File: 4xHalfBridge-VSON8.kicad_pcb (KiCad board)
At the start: 2 copper layers, 90 x 36 mm, 98 parts, among them U1 VSON8_Nexfet, U10 24LC01, U2 VSON8_Nexfet, U3 VSON8_Nexfet, U4 VSON8_Nexfet, U5 VSON8_Nexfet, U6 VSON8_Nexfet, U7 VSON8_Nexfet, U8 VSON8_Nexfet, U9 PowerStage_L

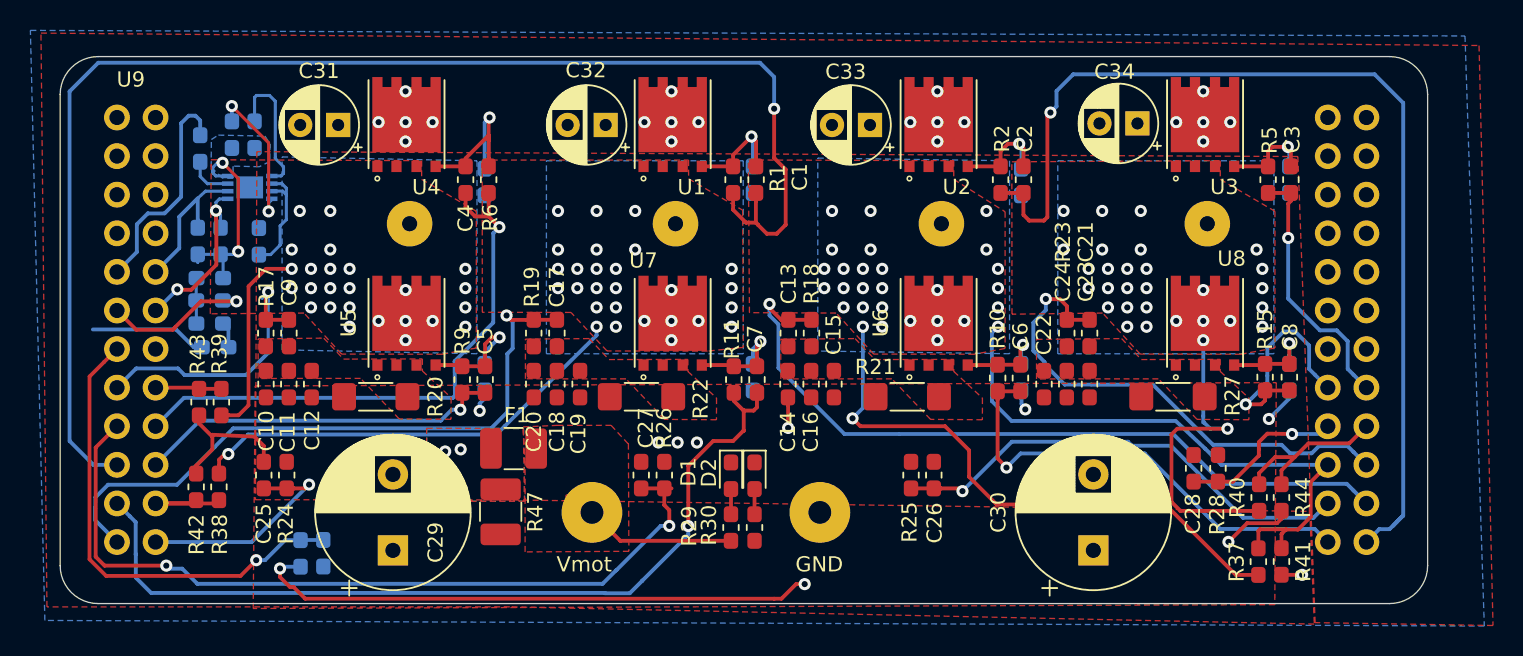
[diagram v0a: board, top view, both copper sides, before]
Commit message: add files
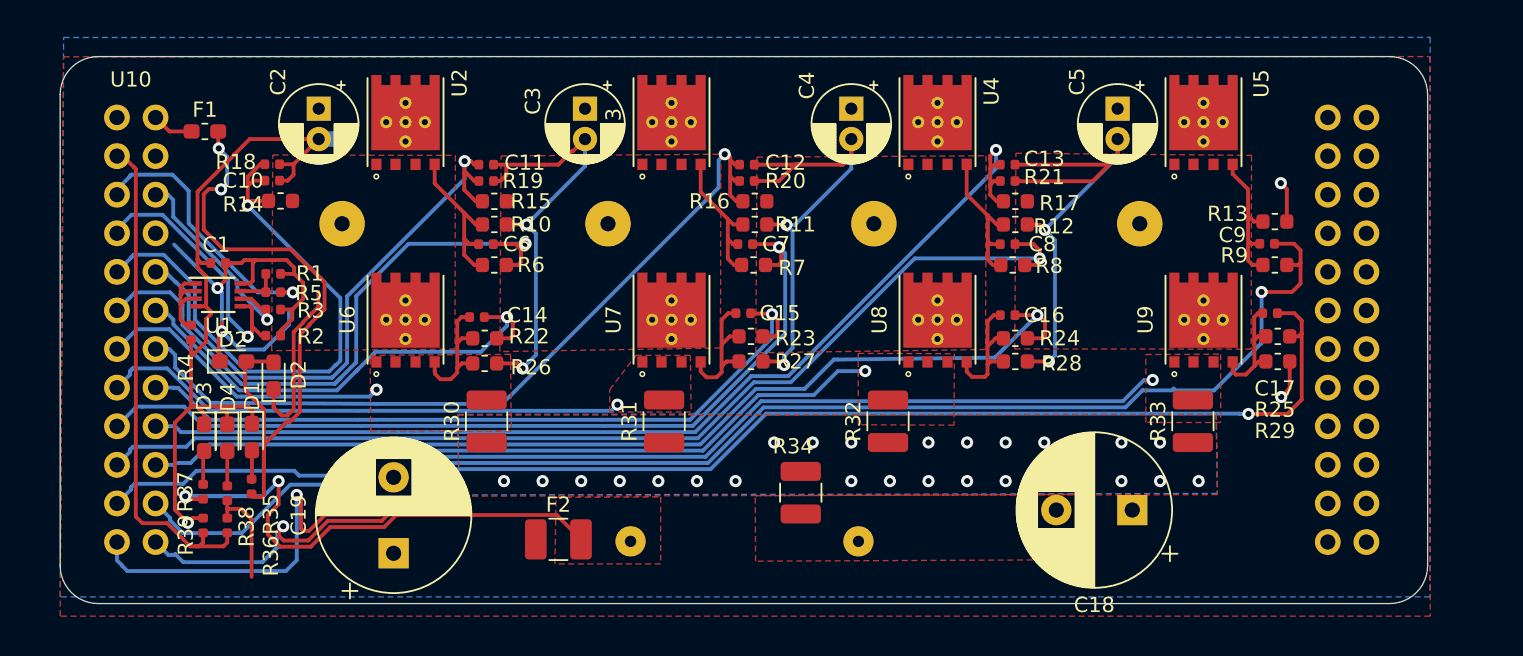
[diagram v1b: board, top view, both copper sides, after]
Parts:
- removed C20, C21, C22, C23, C24, C25, C26, C27, C28: C, Capacitor_SMD:C_0603_1608Metric_Pad1.05x0.95mm_HandSolder
- removed C29, C30: CP, Capacitor_THT:CP_Radial_D10.0mm_P5.00mm
- removed C31, C32, C33, C34: CP, Capacitor_THT:CP_Radial_D5.0mm_P2.50mm
- removed C35: X7R, 47-nF, Capacitor_SMD:C_0603_1608Metric_Pad1.05x0.95mm_HandSolder
- removed the D2 at (45.7, 27.6)
- removed R40, R41, R42, R43, R44, R45, R46: R, Resistor_SMD:R_0603_1608Metric_Pad1.05x0.95mm_HandSolder
- removed R47: R, Resistor_SMD:R_1210_3225Metric_Pad1.42x2.65mm_HandSolder
- removed the U10 at (12.5, 8.61)
- added D2: D_Schottky, Diode_SMD:D_0603_1608Metric_Pad1.05x0.95mm_HandSolder, F.Cu at (14.0, 21.0)
- added D2: D_Schottky, Diode_SMD:D_0603_1608Metric_Pad1.05x0.95mm_HandSolder, F.Cu at (11.4, 20.1)
- added U9: VSON8_Nexfet, Custom_Mosfet:MOSFET_CSD19531Q5A, F.Cu at (75.2, 17.3)
- C1, C10, C11, C12, C13, C14, C15, C16, C17, C6, C7, C8, C9: footprint Capacitor_SMD:C_0603_1608Metric_Pad1.05x0.95mm_HandSolder -> Capacitor_SMD:C_0402_1005Metric
- C18, C19: value C -> CP; footprint Capacitor_SMD:C_0603_1608Metric_Pad1.05x0.95mm_HandSolder -> Capacitor_THT:CP_Radial_D10.0mm_P5.00mm
- C2, C3, C4, C5: footprint Capacitor_SMD:C_0603_1608Metric_Pad1.05x0.95mm_HandSolder -> Capacitor_THT:CP_Radial_D5.0mm_P2.00mm
- D3: moved to F.Cu
- D4: value D_Schottky -> LED; footprint Diode_SMD:D_0603_1608Metric_Pad1.05x0.95mm_HandSolder -> LED_SMD:LED_0603_1608Metric_Pad1.05x0.95mm_HandSolder; moved to F.Cu
- F1: footprint Fuse:Fuse_1210_3225Metric_Pad1.42x2.65mm_HandSolder -> Fuse:Fuse_0603_1608Metric_Pad1.05x0.95mm_HandSolder
- F2: footprint Fuse:Fuse_0603_1608Metric_Pad1.05x0.95mm_HandSolder -> Fuse:Fuse_1210_3225Metric_Pad1.42x2.65mm_HandSolder; moved to F.Cu
- R1, R18, R19, R2, R37, R38, R39, R5: value R -> R_Small; footprint Resistor_SMD:R_0603_1608Metric_Pad1.05x0.95mm_HandSolder -> Resistor_SMD:R_0402_1005Metric
- R10, R11, R15, R17, R23, R24, R25, R26, R28, R29, R6, R9: value R -> R_Small; footprint Resistor_SMD:R_0603_1608Metric_Pad1.05x0.95mm_HandSolder -> Resistor_SMD:R_0603_1608Metric
- R12, R13, R14, R16, R7, R8: value R -> R_Small; footprint Resistor_SMD:R_0603_1608Metric_Pad1.05x0.95mm_HandSolder -> Resistor_SMD:R_0603_1608Metric; moved to F.Cu
- R20, R21: value R -> R_Small; footprint Resistor_SMD:R_1806_4516Metric_Pad1.57x1.80mm_HandSolder -> Resistor_SMD:R_0402_1005Metric
- R22, R27: value R -> R_Small; footprint Resistor_SMD:R_1806_4516Metric_Pad1.57x1.80mm_HandSolder -> Resistor_SMD:R_0603_1608Metric
- R3, R35, R36, R4: value R -> R_Small; footprint Resistor_SMD:R_0603_1608Metric_Pad1.05x0.95mm_HandSolder -> Resistor_SMD:R_0402_1005Metric; moved to F.Cu
- R30: value R -> R_Small; footprint Resistor_SMD:R_0603_1608Metric_Pad1.05x0.95mm_HandSolder -> Resistor_SMD:R_1210_3225Metric
- R31, R32, R33, R34: value R -> R_Small; footprint Resistor_SMD:R_0603_1608Metric_Pad1.05x0.95mm_HandSolder -> Resistor_SMD:R_1210_3225Metric; moved to F.Cu
- U1: value VSON8_Nexfet -> 24LC01; footprint Custom_Mosfet:MOSFET_CSD19531Q5A -> Package_DFN_QFN:DFN-8-1EP_3x2mm_P0.5mm_EP1.75x1.45mm
- moved R37 69.6 mm to (9.41, 28.6)
- moved R5 65.9 mm to (14.0, 15.5), turned to 180 degrees
- moved R33 65.1 mm to (74.5, 24.0)
- moved C9 64.7 mm to (79.4, 12.3), turned to 180 degrees
- moved R4 55.5 mm to (8.61, 18.2)
- moved U5 54.1 mm to (75.2, 4.32)
- moved R9 54.0 mm to (79.9, 13.7), turned to 180 degrees
- moved R15 52.0 mm to (28.6, 9.53), turned to 180 degrees
- moved R17 50.1 mm to (62.9, 9.53), turned to 0 degrees
- moved R2 49.0 mm to (14.0, 18.4), turned to 180 degrees
- moved R24 48.8 mm to (62.9, 18.5), turned to 0 degrees
- moved C17 47.0 mm to (79.6, 16.9), turned to 180 degrees
- moved C3 46.7 mm to (34.5, 3.43)
- moved C2 46.6 mm to (17.0, 3.43)
- moved R32 45.8 mm to (54.5, 24.0)
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- renumbered U9 to U10
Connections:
- C1 pad 1: Net-(C1-Pad1) -> /CarrierBoard/5V
- C1 pad 2: /BHG -> GND
- C10 pad 2: Net-(C10-Pad2) -> /4xHalfBridge/VSENA
- C11 pad 2: Net-(C10-Pad2) -> /4xHalfBridge/VSENB
- C12 pad 2: Net-(C10-Pad2) -> /4xHalfBridge/VSENC
- C13 pad 1: Net-(C13-Pad1) -> GND
- C13 pad 2: /CISENP -> /4xHalfBridge/VSEND
- C14 pad 1: GND -> /4xHalfBridge/ALG
- C14 pad 2: Net-(C13-Pad1) -> Net-(C14-Pad2)
- C15 pad 1: GND -> /4xHalfBridge/BLG
- C15 pad 2: Net-(C13-Pad1) -> Net-(C15-Pad2)
- C16 pad 1: GND -> /4xHalfBridge/CLG
- C16 pad 2: Net-(C13-Pad1) -> Net-(C16-Pad2)
- C17 pad 1: Net-(C17-Pad1) -> /4xHalfBridge/DLG
- C17 pad 2: /BISENP -> Net-(C17-Pad2)
- C18 pad 1: GND -> /4xHalfBridge/VMOT
- C18 pad 2: Net-(C17-Pad1) -> GND
- C19 pad 1: GND -> /4xHalfBridge/VMOT
- C19 pad 2: Net-(C17-Pad1) -> GND
- C2 pad 1: Net-(C2-Pad1) -> /4xHalfBridge/VMOT
- C2 pad 2: /CHG -> GND
- C3 pad 1: Net-(C3-Pad1) -> /4xHalfBridge/VMOT
- C3 pad 2: /DHG -> GND
- C4 pad 1: Net-(C4-Pad1) -> /4xHalfBridge/VMOT
- C4 pad 2: /AHG -> GND
- C5 pad 1: Net-(C5-Pad1) -> /4xHalfBridge/VMOT
- C5 pad 2: /ALG -> GND
- C6 pad 1: Net-(C6-Pad1) -> /4xHalfBridge/AHG
- C6 pad 2: /CLG -> Net-(C6-Pad2)
- C7 pad 1: Net-(C7-Pad1) -> /4xHalfBridge/BHG
- C7 pad 2: /BLG -> Net-(C7-Pad2)
- C8 pad 1: Net-(C8-Pad1) -> /4xHalfBridge/CHG
- C8 pad 2: /DLG -> Net-(C8-Pad2)
- C9 pad 1: Net-(C10-Pad2) -> /4xHalfBridge/DHG
- C9 pad 2: /AISENP -> Net-(C9-Pad2)
- D4 pad 1: Net-(C35-Pad1) -> GND
- F1 pad 1: /MISENP -> /CarrierBoard/5V_IN_RAW
- F1 pad 2: VCC -> Net-(D2-Pad2)
- F2 pad 1: /5V -> /4xHalfBridge/VMOT
- F2 pad 2: Net-(D4-Pad2) -> VCC
- R1 pad 1: Net-(C1-Pad1) -> Net-(R1-Pad1)
- R1 pad 2: /BHG -> /CarrierBoard/5V
- R10 pad 1: Net-(C6-Pad1) -> Net-(C6-Pad2)
- R10 pad 2: /CLG -> GND
- R11 pad 1: Net-(C7-Pad1) -> Net-(C7-Pad2)
- R11 pad 2: /BLG -> GND
- R12 pad 1: Net-(C5-Pad1) -> GND
- R12 pad 2: GND -> Net-(C8-Pad2)
- R13 pad 1: Net-(C6-Pad1) -> Net-(C9-Pad2)
- R14 pad 1: Net-(C7-Pad1) -> Net-(R14-Pad1)
- R14 pad 2: GND -> /4xHalfBridge/VSENA
- R15 pad 1: Net-(C8-Pad1) -> Net-(R15-Pad1)
- R15 pad 2: /DLG -> /4xHalfBridge/VSENB
- R16 pad 1: Net-(C8-Pad1) -> Net-(R16-Pad1)
- R16 pad 2: GND -> /4xHalfBridge/VSENC
- R17 pad 1: Net-(C10-Pad2) -> /4xHalfBridge/VSEND
- R17 pad 2: /AISENP -> Net-(R17-Pad2)
- R18 pad 1: Net-(C13-Pad1) -> GND
- R18 pad 2: /CISENP -> /4xHalfBridge/VSENA
- R19 pad 1: Net-(C17-Pad1) -> GND
- R19 pad 2: /BISENP -> /4xHalfBridge/VSENB
- R2 pad 1: Net-(C2-Pad1) -> /CarrierBoard/5V
- R2 pad 2: /CHG -> /CarrierBoard/EEPROM_SDA
- R20 pad 1: Net-(C10-Pad2) -> GND
- R20 pad 2: GND -> /4xHalfBridge/VSENC
- R21 pad 1: Net-(C13-Pad1) -> GND
- R21 pad 2: GND -> /4xHalfBridge/VSEND
- R22 pad 1: Net-(C17-Pad1) -> /4xHalfBridge/ALG
- R22 pad 2: GND -> Net-(C14-Pad2)
- R23 pad 1: Net-(C21-Pad1) -> /4xHalfBridge/BLG
- R23 pad 2: /DISENP -> Net-(C15-Pad2)
- R24 pad 1: GND -> Net-(C16-Pad2)
- R24 pad 2: /AISENN -> /4xHalfBridge/CLG
- R25 pad 1: GND -> /4xHalfBridge/DLG
- R25 pad 2: /CISENN -> Net-(C17-Pad2)
- R26 pad 1: GND -> Net-(C14-Pad2)
- R26 pad 2: /BISENN -> GND
- R27 pad 1: Net-(C21-Pad1) -> Net-(C15-Pad2)
- R28 pad 1: GND -> Net-(C16-Pad2)
- R28 pad 2: /DISENN -> GND
- R29 pad 1: Net-(D1-Pad2) -> Net-(C17-Pad2)
- R29 pad 2: VCC -> GND
- R3 pad 1: Net-(C1-Pad1) -> /CarrierBoard/5V
- R3 pad 2: GND -> /CarrierBoard/EEPROM_SCL
- R30 pad 1: Net-(D2-Pad2) -> /4xHalfBridge/AISENN
- R30 pad 2: /MISENN -> /4xHalfBridge/AISENP
- R31 pad 1: Net-(D3-Pad2) -> /4xHalfBridge/AISENN
- R31 pad 2: Net-(D4-Pad2) -> /4xHalfBridge/BISENP
- R32 pad 1: Net-(C35-Pad1) -> /4xHalfBridge/AISENN
- R32 pad 2: Net-(R32-Pad2) -> /4xHalfBridge/CISENP
- R33 pad 1: Net-(C35-Pad1) -> /4xHalfBridge/AISENN
- R33 pad 2: /SDA -> /4xHalfBridge/DISENP
- R34 pad 1: Net-(C35-Pad1) -> GND
- R34 pad 2: /SCL -> /4xHalfBridge/AISENN
- R35 pad 1: /WP -> Net-(D2-Pad2)
- R35 pad 2: Net-(R35-Pad2) -> Net-(D1-Pad2)
- R36 pad 1: Net-(R36-Pad1) -> /4xHalfBridge/VMOT
- R36 pad 2: GND -> /CarrierBoard/VSEN_VMOT
- R37 pad 1: /C -> VCC
- R37 pad 2: /VSENC -> Net-(D3-Pad2)
- R38 pad 1: /B -> /4xHalfBridge/VMOT
- R38 pad 2: /VSENB -> Net-(D4-Pad2)
- R39 pad 1: /A -> /CarrierBoard/VSEN_VMOT
- R39 pad 2: /VSENA -> GND
- R4 pad 1: Net-(C2-Pad1) -> Net-(R4-Pad1)
- R5 pad 1: Net-(C3-Pad1) -> /CarrierBoard/EEPROM_WP
- R5 pad 2: /DHG -> Net-(R1-Pad1)
- R6 pad 1: Net-(C4-Pad1) -> /4xHalfBridge/AHG
- R6 pad 2: /AHG -> Net-(C6-Pad2)
- R7 pad 1: Net-(C3-Pad1) -> /4xHalfBridge/BHG
- R7 pad 2: GND -> Net-(C7-Pad2)
- R8 pad 1: Net-(C4-Pad1) -> Net-(C8-Pad2)
- R8 pad 2: GND -> /4xHalfBridge/CHG
- R9 pad 1: Net-(C5-Pad1) -> /4xHalfBridge/DHG
- R9 pad 2: /ALG -> Net-(C9-Pad2)
- U1 pad 1: /B -> Net-(R4-Pad1)
- U1 pad 2: Net-(C1-Pad1) -> Net-(R4-Pad1)
- U1 pad 3: /MISENN -> Net-(R4-Pad1)
- U10 pad 10: /SCL -> /4xHalfBridge/VSENB
- U10 pad 11: /5V -> /4xHalfBridge/AHG
- U10 pad 12: /SDA -> /4xHalfBridge/ALG
- U10 pad 13: /VSEN_VMOT -> /4xHalfBridge/AISENP
- U10 pad 14: Net-(U9-Pad14) -> /4xHalfBridge/VSENC
- U10 pad 15: /AISENP -> /4xHalfBridge/BISENP
- U10 pad 16: /VSENA -> /4xHalfBridge/BLG
- U10 pad 17: /BISENN -> /4xHalfBridge/BHG
- U10 pad 18: /AHG -> /4xHalfBridge/VSEND
- U10 pad 19: /BHG -> /4xHalfBridge/CHG
- U10 pad 2: Net-(U9-Pad2) -> /CarrierBoard/5V_IN_RAW
- U10 pad 20: /ALG -> /4xHalfBridge/CLG
- U10 pad 21: /BLG -> /4xHalfBridge/CISENP
- U10 pad 22: /VSENB -> /4xHalfBridge/DISENP
- U10 pad 23: /BISENP -> /4xHalfBridge/DHG
- U10 pad 24: /AISENN -> /4xHalfBridge/DLG
- U10 pad 3: Net-(U9-Pad3) -> /CarrierBoard/VSEN_VMOT
- U10 pad 39: /DLG -> Net-(U10-Pad39)
- U10 pad 40: /DHG -> Net-(U10-Pad40)
- U10 pad 41: /DISENN -> Net-(U10-Pad41)
- U10 pad 42: /VSEND -> Net-(U10-Pad42)
- U10 pad 43: /VSENC -> Net-(U10-Pad43)
- U10 pad 44: /DISENP -> Net-(U10-Pad44)
- U10 pad 45: /CISENN -> Net-(U10-Pad45)
- U10 pad 46: /CISENP -> Net-(U10-Pad46)
- U10 pad 47: /CLG -> Net-(U10-Pad47)
- U10 pad 48: /CHG -> Net-(U10-Pad48)
- U10 pad 5: Net-(U9-Pad5) -> /CarrierBoard/EEPROM_WP
- U10 pad 6: Net-(U9-Pad6) -> /CarrierBoard/EEPROM_SCL
- U10 pad 7: Net-(U9-Pad7) -> /CarrierBoard/EEPROM_SDA
- U10 pad 9: /WP -> /4xHalfBridge/VSENA
- U2 pad 1: /C -> Net-(R14-Pad1)
- U2 pad 2: Net-(C2-Pad1) -> Net-(C6-Pad2)
- U2 pad 3: /MISENN -> /4xHalfBridge/VMOT
- U3 pad 1: /D -> Net-(R15-Pad1)
- U3 pad 2: Net-(C3-Pad1) -> Net-(C7-Pad2)
- U3 pad 3: /MISENN -> /4xHalfBridge/VMOT
- U4 pad 1: /A -> Net-(R16-Pad1)
- U4 pad 2: Net-(C4-Pad1) -> Net-(C8-Pad2)
- U4 pad 3: /MISENN -> /4xHalfBridge/VMOT
- U5 pad 1: Net-(C10-Pad2) -> Net-(R17-Pad2)
- U5 pad 2: Net-(C5-Pad1) -> Net-(C9-Pad2)
- U5 pad 3: /A -> /4xHalfBridge/VMOT
- U6 pad 1: Net-(C13-Pad1) -> /4xHalfBridge/AISENP
- U6 pad 2: Net-(C6-Pad1) -> Net-(C14-Pad2)
- U6 pad 3: /C -> Net-(R14-Pad1)
- U7 pad 1: Net-(C17-Pad1) -> /4xHalfBridge/BISENP
- U7 pad 2: Net-(C7-Pad1) -> Net-(C15-Pad2)
- U7 pad 3: /B -> Net-(R15-Pad1)
- U8 pad 1: Net-(C21-Pad1) -> /4xHalfBridge/CISENP
- U8 pad 2: Net-(C8-Pad1) -> Net-(C16-Pad2)
- U8 pad 3: /D -> Net-(R16-Pad1)
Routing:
- net GND: track 40.6 -> 151.4 mm, vias 11 -> 9
- net /4xHalfBridge/DHG: track 0.00 -> 100.7 mm, vias 0 -> 3
- net /BHG: track 91.8 -> 0.00 mm, vias 1 -> 0
- net /4xHalfBridge/DLG: track 0.00 -> 90.6 mm, vias 0 -> 3
- net /4xHalfBridge/DISENP: track 0.00 -> 70.7 mm, vias 0 -> 1
- net /4xHalfBridge/CHG: track 0.00 -> 70.3 mm, vias 0 -> 1
- net /4xHalfBridge/VSEND: track 0.00 -> 70.0 mm, vias 0 -> 1
- net /CHG: track 68.5 -> 0.00 mm, vias 1 -> 0
- net /4xHalfBridge/CLG: track 0.00 -> 66.4 mm, vias 0 -> 1
- net /BLG: track 57.7 -> 0.00 mm, vias 1 -> 0
- net /4xHalfBridge/BHG: track 0.00 -> 57.4 mm, vias 0 -> 1
- net /BISENN: track 53.8 -> 0.00 mm, vias 2 -> 0
- net /4xHalfBridge/CISENP: track 0.00 -> 53.2 mm, vias 0 -> 1
- net /4xHalfBridge/VSENC: track 0.00 -> 52.8 mm, vias 0 -> 1
- net /CISENP: track 50.2 -> 0.00 mm, vias 1 -> 0
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- added copper zone on B.Cu, net /4xHalfBridge/AISENN
- added copper zone on F.Cu, net /4xHalfBridge/AISENN
- added copper zone on F.Cu, net /4xHalfBridge/AISENP
- added copper zone on F.Cu, net /4xHalfBridge/BISENP
- added copper zone on F.Cu, net /4xHalfBridge/CISENP
- added copper zone on F.Cu, net /4xHalfBridge/DISENP
- added copper zone on F.Cu, net /4xHalfBridge/VMOT
- added copper zone on F.Cu, net Net-(R14-Pad1)
- added copper zone on F.Cu, net Net-(R15-Pad1)
- added copper zone on F.Cu, net Net-(R16-Pad1)
- added copper zone on F.Cu, net Net-(R17-Pad2)
- removed copper zone on B.Cu, net /A
- removed copper zone on F.Cu, net /A
- removed copper zone on B.Cu, net /B
- removed copper zone on F.Cu, net /B
- removed copper zone on B.Cu, net /C
- removed copper zone on F.Cu, net /C
- removed copper zone on B.Cu, net /D
- removed copper zone on F.Cu, net /D
- removed copper zone on F.Cu, net /MISENN
- removed copper zone on B.Cu, net /MISENP
- removed copper zone on F.Cu, net /MISENP
- removed copper zone on F.Cu, net Net-(C10-Pad2)
- removed copper zone on F.Cu, net Net-(C13-Pad1)
- removed copper zone on F.Cu, net Net-(C17-Pad1)
- removed copper zone on F.Cu, net Net-(C21-Pad1)
- removed copper zone on B.Cu, net Net-(C35-Pad1)
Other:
- board text removed: "GND"
- board text removed: "Vmot"
